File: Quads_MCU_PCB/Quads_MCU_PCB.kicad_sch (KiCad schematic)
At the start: 106 parts, among them J1 USB_C_Receptacle_USB2.0_16P, J2 Conn_01x06_Pin, J3 Conn_01x02_Pin, J4 Conn_01x04_Pin, J5 Conn_01x04_Pin, J6 Conn_01x04_Pin, J7 Conn_01x04_Pin, SW1 SW_Push, U1 STM32H723ZGTx, U10 BMI088, U3 ADM3057ExRW, U4 TSR_1-2450, U5 AP7361C-33E, U6 ADM3057ExRW, U7 ADM3057ExRW, U8 MCP2518FD-xQBB, U9 ADM3057ExRW, Y1 40MHz, Y2 25MHz

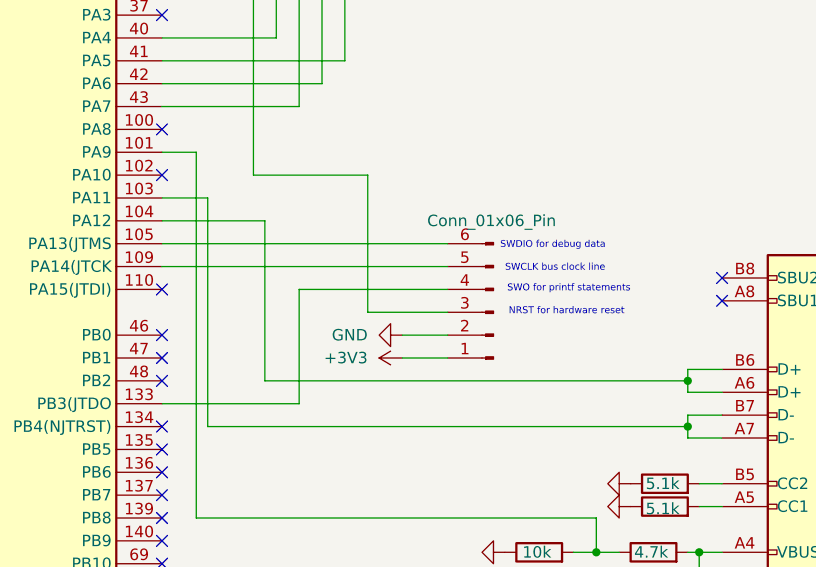
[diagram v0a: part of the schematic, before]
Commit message: Fixed debug pin order
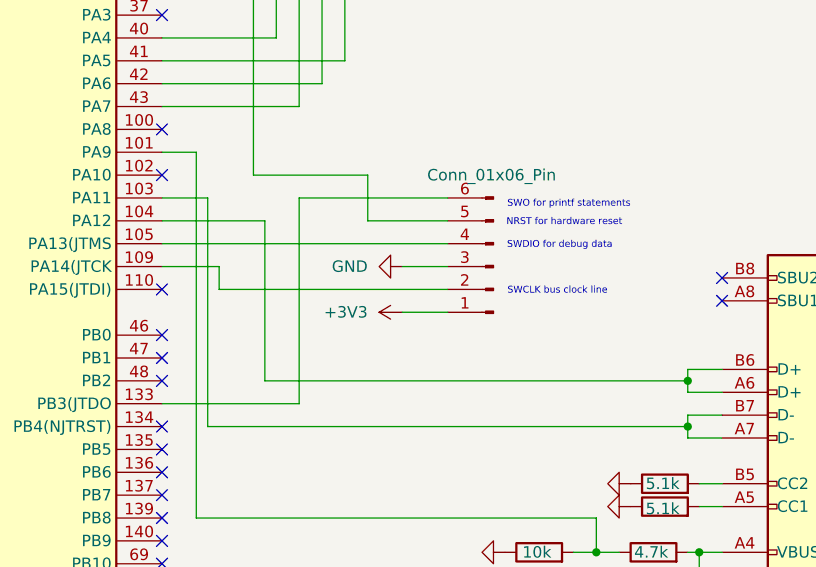
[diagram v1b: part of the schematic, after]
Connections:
- net GND: now also J2.3 (Pin_3); no longer J2.2 (Pin_2)
- net at C1.2, U1.25 (NRST): now also J2.5 (Pin_5); no longer J2.3 (Pin_3)
- net at J2.4 (Pin_4): now also U1.105 (PA13(JTMS); no longer U1.133 (PB3(JTDO)
- net at U1.109 (PA14(JTCK): now also J2.2 (Pin_2); no longer J2.5 (Pin_5)
- net at J2.6 (Pin_6): now also U1.133 (PB3(JTDO); no longer U1.105 (PA13(JTMS)
